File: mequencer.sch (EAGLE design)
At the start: 58 parts, among them IC1 NE555D, IC10 LF353D, IC11 NE555D, IC12 NE555D, IC2 4163D, IC3 74HC85D, IC4 4051D, IC5 4051D, IC6 74HCT04D, IC7 4051D, IC8 4051D, IC9 LF353D

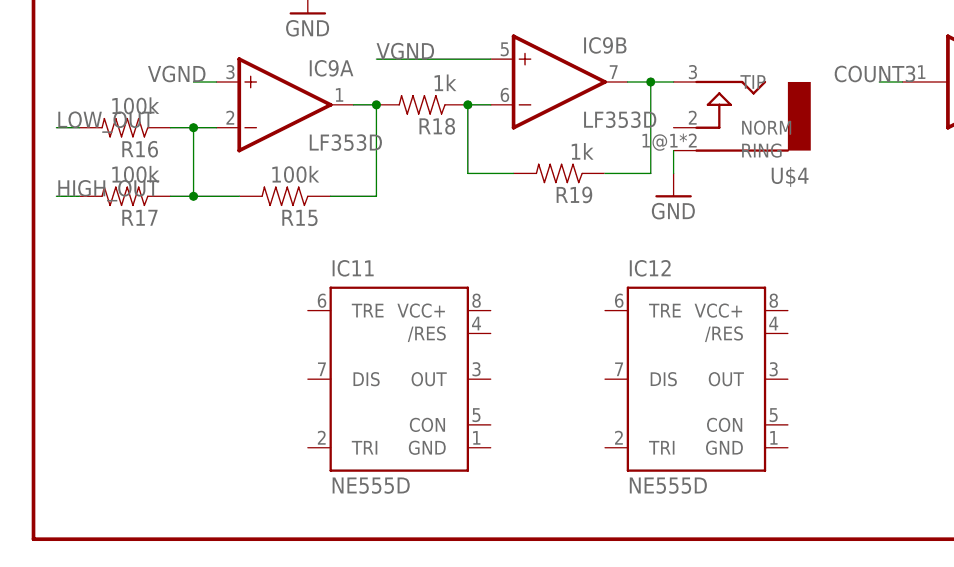
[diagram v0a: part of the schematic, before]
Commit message: 55555555555555555
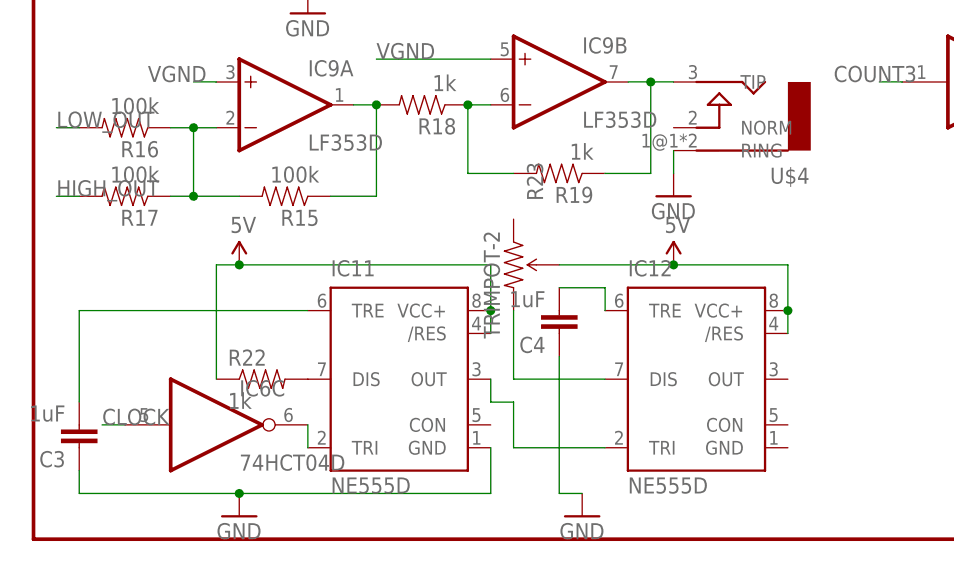
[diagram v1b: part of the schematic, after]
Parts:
- added C3, C4: 1uF, SparkFun-Capacitors:CAP0603-CAP
- added R22: 1k, SparkFun-Resistors:RESISTOR0603
- added R23: TRIMPOT-2, SparkFun-Electromechanical:TRIMPOT-2
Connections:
- new net N$16: IC11.DIS, R22.2
- new net N$17: IC12.DIS, R23.CW
- new net N$18: C3.2, IC11.TRE
- new net N$20: IC11.TRI, IC6C.O
- new net N$21: C4.2, IC12.TRE
- new net N$23: IC11.OUT, IC12.TRI
- net 5V: now also IC11./RES, IC11.VCC+, IC12./RES, IC12.VCC+, R22.1, R23.WIPER
- net CLOCK: now also IC6C.I
- net GND: now also C3.1, C4.1, IC11.GND
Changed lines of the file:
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@@
 <part name="IC11" library="SparkFun-AnalogIC" deviceset="NE555" device="D"/>
 <part name="IC12" library="SparkFun-AnalogIC" deviceset="NE555" device="D"/>
+<part name="R22" library="SparkFun-Resistors" deviceset="RESISTOR" device="0603" value="1k"/>
+<part name="SUPPLY8" library="SparkFun-Aesthetics" deviceset="5V" device=""/>
+<part name="GND11" library="SparkFun-Aesthetics" deviceset="GND" device=""/>
+<part name="C3" library="SparkFun-Capacitors" deviceset="CAP" device="0603-CAP" value="1uF"/>
+<part name="GND12" library="SparkFun-Aesthetics" deviceset="GND" device=""/>
+<part name="C4" library="SparkFun-Capacitors" deviceset="CAP" device="0603-CAP" value="1uF"/>
+<part name="SUPPLY9" library="SparkFun-Aesthetics" deviceset="5V" device=""/>
+<part name="R23" library="SparkFun-Electromechanical" deviceset="TRIMPOT" device="-2"/>
 </parts>
 <sheets>
@@
 <instance part="IC11" gate="G$1" x="40.64" y="17.78"/>
 <instance part="IC12" gate="G$1" x="73.66" y="17.78"/>
+<instance part="R22" gate="G$1" x="25.4" y="17.78"/>
+<instance part="SUPPLY8" gate="G$1" x="22.86" y="30.48"/>
+<instance part="GND11" gate="1" x="22.86" y="2.54"/>
+<instance part="C3" gate="G$1" x="5.08" y="12.7" rot="R180"/>
+<instance part="IC6" gate="C" x="20.32" y="12.7"/>
+<instance part="GND12" gate="1" x="60.96" y="2.54"/>
+<instance part="C4" gate="G$1" x="58.42" y="25.4" rot="R180"/>
+<instance part="SUPPLY9" gate="G$1" x="71.12" y="30.48"/>
+<instance part="R23" gate="R?" x="53.34" y="30.48" rot="R270"/>
 </instances>
 <busses>
@@
 <wire x1="30.48" y1="86.36" x2="33.02" y2="86.36" width="0.1524" layer="91"/>
 </segment>
+<segment>
+<pinref part="SUPPLY8" gate="G$1" pin="5V"/>
+<wire x1="22.86" y1="30.48" x2="50.8" y2="30.48" width="0.1524" layer="91"/>
+<pinref part="R22" gate="G$1" pin="1"/>
+<wire x1="20.32" y1="17.78" x2="20.32" y2="30.48" width="0.1524" layer="91"/>
+<wire x1="20.32" y1="30.48" x2="22.86" y2="30.48" width="0.1524" layer="91"/>
+<junction x="22.86" y="30.48"/>
+<pinref part="IC11" gate="G$1" pin="/RES"/>
+<pinref part="IC11" gate="G$1" pin="VCC+"/>
+<wire x1="50.8" y1="22.86" x2="50.8" y2="25.4" width="0.1524" layer="91"/>
+<wire x1="50.8" y1="25.4" x2="50.8" y2="30.48" width="0.1524" layer="91"/>
+<junction x="50.8" y="25.4"/>
+</segment>
+<segment>
+<pinref part="R23" gate="R?" pin="WIPER"/>
+<pinref part="SUPPLY9" gate="G$1" pin="5V"/>
+<wire x1="58.42" y1="30.48" x2="71.12" y2="30.48" width="0.1524" layer="91"/>
+<pinref part="IC12" gate="G$1" pin="/RES"/>
+<pinref part="IC12" gate="G$1" pin="VCC+"/>
+<wire x1="83.82" y1="22.86" x2="83.82" y2="25.4" width="0.1524" layer="91"/>
+<wire x1="83.82" y1="25.4" x2="83.82" y2="30.48" width="0.1524" layer="91"/>
+<junction x="83.82" y="25.4"/>
+<wire x1="83.82" y1="30.48" x2="71.12" y2="30.48" width="0.1524" layer="91"/>
+<junction x="71.12" y="30.48"/>
+</segment>
 </net>
 <net name="N$1" class="0">
@@
 <wire x1="30.48" y1="63.5" x2="30.48" y2="60.96" width="0.1524" layer="91"/>
 </segment>
+<segment>
+<pinref part="IC11" gate="G$1" pin="GND"/>
+<wire x1="50.8" y1="10.16" x2="50.8" y2="5.08" width="0.1524" layer="91"/>
+<pinref part="GND11" gate="1" pin="GND"/>
+<wire x1="50.8" y1="5.08" x2="22.86" y2="5.08" width="0.1524" layer="91"/>
+<junction x="22.86" y="5.08"/>
+<pinref part="C3" gate="G$1" pin="1"/>
+<wire x1="22.86" y1="5.08" x2="5.08" y2="5.08" width="0.1524" layer="91"/>
+<wire x1="5.08" y1="5.08" x2="5.08" y2="7.62" width="0.1524" layer="91"/>
+</segment>
+<segment>
+<pinref part="C4" gate="G$1" pin="1"/>
+<wire x1="58.42" y1="20.32" x2="58.42" y2="5.08" width="0.1524" layer="91"/>
+<pinref part="GND12" gate="1" pin="GND"/>
+<wire x1="58.42" y1="5.08" x2="60.96" y2="5.08" width="0.1524" layer="91"/>
+</segment>
 </net>
 <net name="N$2" class="0">
@@
 <wire x1="17.78" y1="99.06" x2="2.54" y2="99.06" width="0.1524" layer="91"/>
 <label x="2.54" y="99.06" size="1.778" layer="95"/>
+</segment>
+<segment>
+<pinref part="IC6" gate="C" pin="I"/>
+<wire x1="10.16" y1="12.7" x2="7.62" y2="12.7" width="0.1524" layer="91"/>
+<label x="7.62" y="12.7" size="1.778" layer="95"/>
 </segment>
 </net>
@@
 </segment>
 </net>
+<net name="N$16" class="0">
+<segment>
+<pinref part="IC11" gate="G$1" pin="DIS"/>
+<pinref part="R22" gate="G$1" pin="2"/>
+</segment>
+</net>
+<net name="N$18" class="0">
+<segment>
+<pinref part="IC11" gate="G$1" pin="TRE"/>
+<pinref part="C3" gate="G$1" pin="2"/>
+<wire x1="5.08" y1="15.24" x2="5.08" y2="25.4" width="0.1524" layer="91"/>
+<wire x1="5.08" y1="25.4" x2="30.48" y2="25.4" width="0.1524" layer="91"/>
+</segment>
+</net>
+<net name="N$20" class="0">
+<segment>
+<pinref part="IC6" gate="C" pin="O"/>
+<pinref part="IC11" gate="G$1" pin="TRI"/>
+<wire x1="30.48" y1="12.7" x2="30.48" y2="10.16" width="0.1524" layer="91"/>
+</segment>
+</net>
+<net name="N$17" class="0">
+<segment>
+<pinref part="R23" gate="R?" pin="CW"/>
+<wire x1="53.34" y1="25.4" x2="53.34" y2="17.78" width="0.1524" layer="91"/>
+<pinref part="IC12" gate="G$1" pin="DIS"/>
+<wire x1="53.34" y1="17.78" x2="63.5" y2="17.78" width="0.1524" layer="91"/>
+</segment>
+</net>
+<net name="N$21" class="0">
+<segment>
+<pinref part="C4" gate="G$1" pin="2"/>
+<pinref part="IC12" gate="G$1" pin="TRE"/>
+<wire x1="58.42" y1="27.94" x2="63.5" y2="27.94" width="0.1524" layer="91"/>
+<wire x1="63.5" y1="27.94" x2="63.5" y2="25.4" width="0.1524" layer="91"/>
+</segment>
+</net>
+<net name="N$23" class="0">
+<segment>
+<pinref part="IC11" gate="G$1" pin="OUT"/>
+<wire x1="50.8" y1="17.78" x2="50.8" y2="15.24" width="0.1524" layer="91"/>
+<wire x1="50.8" y1="15.24" x2="53.34" y2="15.24" width="0.1524" layer="91"/>
+<wire x1="53.34" y1="15.24" x2="53.34" y2="10.16" width="0.1524" layer="91"/>
+<pinref part="IC12" gate="G$1" pin="TRI"/>
+<wire x1="53.34" y1="10.16" x2="63.5" y2="10.16" width="0.1524" layer="91"/>
+</segment>
+</net>
